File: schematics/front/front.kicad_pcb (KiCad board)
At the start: 4 copper layers, 29.1 x 51.8 mm, 36 parts, among them J1 USB_B_Micro, J2 MOTOR, J3 Conn_01x08_Pin, J6 Conn_02x04_Odd_Even, SW1 RESET, SW2 BOOT, SW3 MODE, U1 LD1117AG-33-AA3-A-R, U2 ESP32-S2-MINI-2-N4, U3 DRV8836

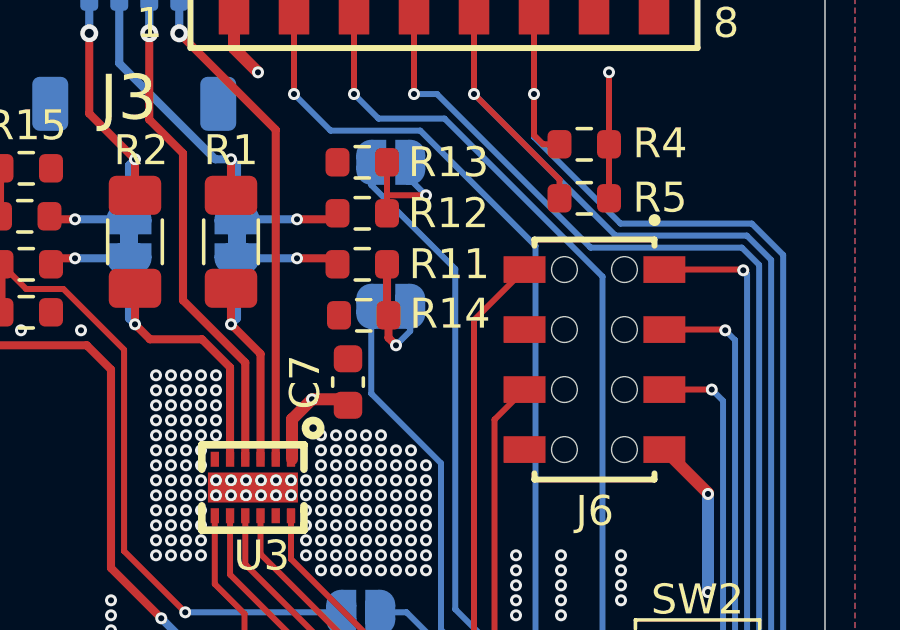
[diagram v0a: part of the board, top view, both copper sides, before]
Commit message: Signed-off-by: Ray33ee <30669752+ray33ee@users.noreply.github.com>
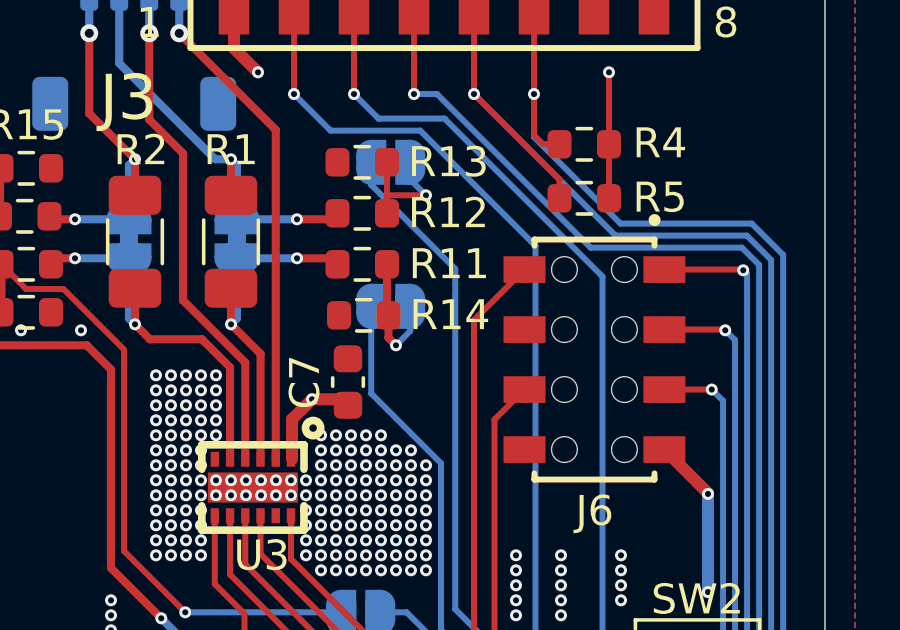
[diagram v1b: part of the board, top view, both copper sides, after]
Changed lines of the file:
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@@
 		(allow_soldermask_bridges_in_footprints no)
 		(tenting front back)
-		(grid_origin 131.05 99)
+		(grid_origin 134.25 87.375)
 		(pcbplotparams
 			(layerselection 0x00000000_00000000_55555555_5755f5ff)
@@
 		(tags "resistor")
 		(property "Reference" "R14"
-			(at -2.875 0.05 0)
+			(at -2.875 0 0)
 			(layer "F.SilkS")
 			(effects
@@
 		(embedded_fonts no)
 	)
+	(gr_rect
+		(start 133.95 86.975)
+		(end 138.05 91.675)
+		(stroke
+			(width 0.1)
+			(type solid)
+		)
+		(fill yes)
+		(layer "F.Mask")
+	)
+	(gr_rect
+		(start 128.15 85.175)
+		(end 130.05 91.075)
+		(stroke
+			(width 0.1)
+			(type solid)
+		)
+		(fill yes)
+		(layer "F.Mask")
+	)
 	(gr_line
